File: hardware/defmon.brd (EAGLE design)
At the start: 50.8 x 48.1 mm, 18 parts, among them IC2 MEGA8-P, Q1 20MHz, X1 MAB5SH, X2 1503_09

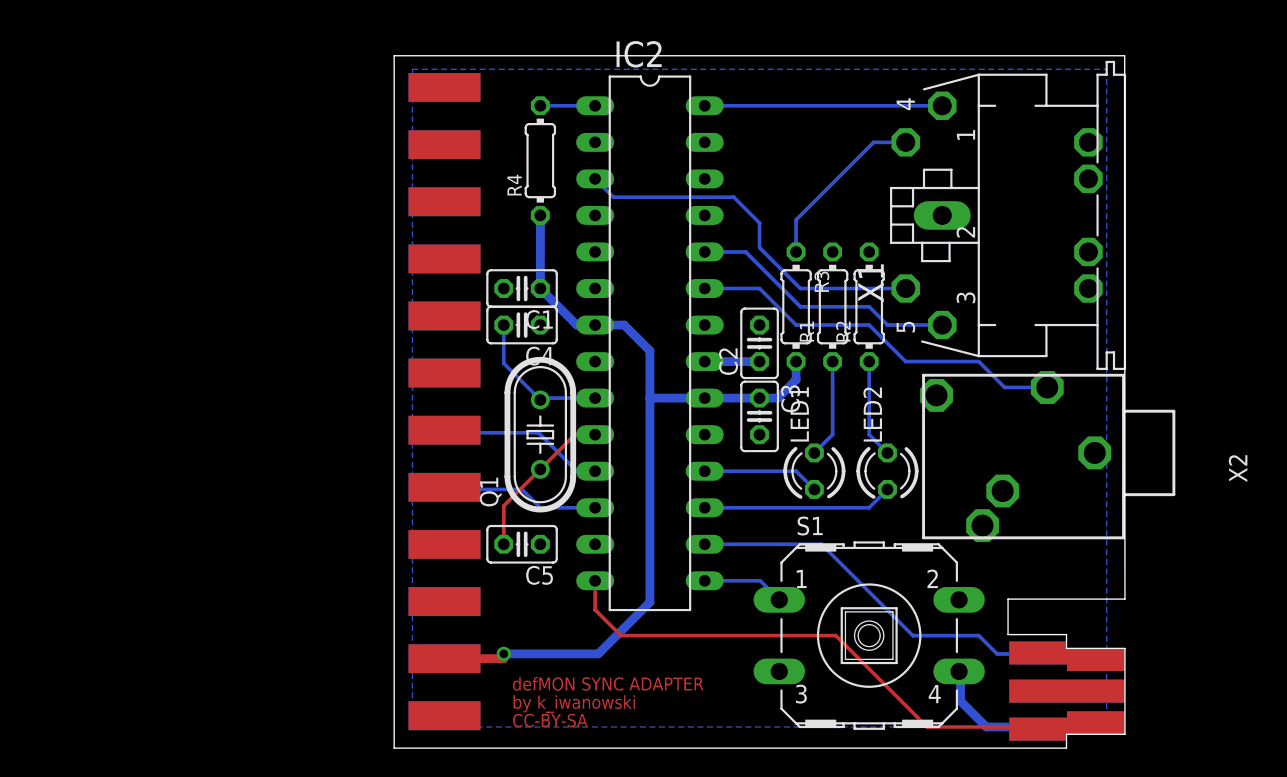
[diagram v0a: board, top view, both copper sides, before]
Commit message: Update cad files
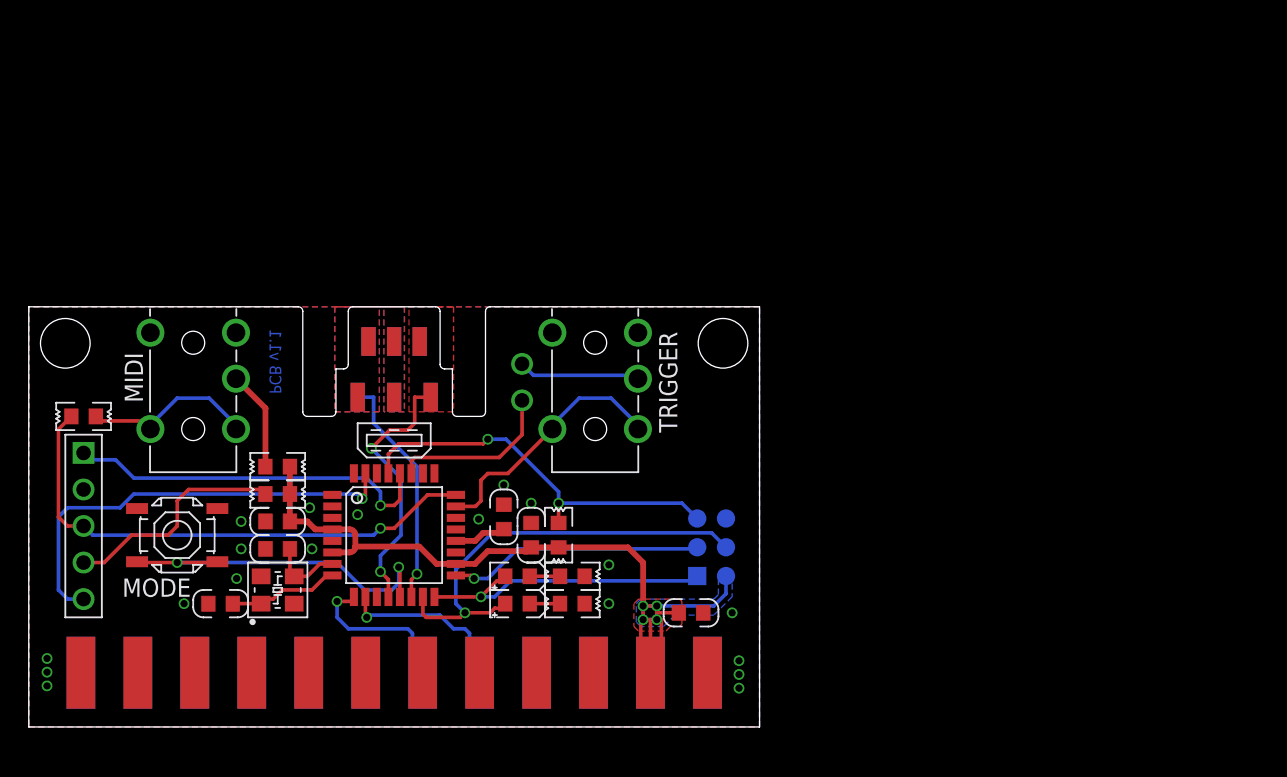
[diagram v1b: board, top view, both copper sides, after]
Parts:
- removed C1: 100nf, rcl:C025-025X050
- removed IC2: MEGA8-P, atmel:DIL28-3
- removed LED1, LED2: (no value), led:LED3MM
- removed S1: (no value), switch-omron:B3F-40XX
- removed X1: MAB5SH, con-hirschmann:MAB5SH
- removed X2: 1503_09, con-lumberg:1503_09
- added C6: 100n, rcl:C0603K
- added CONN2: DNP, GenMDMv2:ICSP_SMD_PROBE
- added CONN3: LINK_PORTFINAL, LinkPort by Jazz:DUAL_BAORD_LINK_FINAL
- added CU: 10uF, rcl:C0603K
- added DIN: 1X5, header by Jazz:1X5
- added IC1: MEGA8-AI_C16190, atmel:TQFP32-08
- added JP1: 2X1, header by Jazz:2X1
- added LED3, LED4: C2286, Led by Jazz:0603K
- added MIDI, TRIG: PJ313, GenMDMv200:PJ313D
- added R5, R6: 220Ohms, rcl:R0603
- added SW1: MODE, Switch by Jazz:TS5215A
- added U$3, U$8: (no value), Mount by Jazz:MOUNT4-40
- added U$9: (no value), Logos by Jazz:CATSKULL_PIXEL_MD
- C2, C3: value 100nf -> 100n; device rcl:C025-025X050 -> rcl:C0603K
- C4, C5: device rcl:C025-025X050 -> rcl:C0603K
- Q1: value 20MHz -> 20MHz_C172730; device crystal:HC49U-V -> GenMDMv200:SX3225
- R1, R2: value 220 -> 220ohms; device rcl:0204/7 -> rcl:R0603
- R3: value 220 -> 220Ohms; device rcl:0204/7 -> rcl:R0603
- R4: value 10k -> 10kOhms; device rcl:0204/7 -> rcl:R0603
- U$1: value GB -> (none); device connector:GB -> Logos by Jazz:JLCJLCJLCJLC
- U$2: value C64U -> CONNECTOR_C64UJ; device connector:C64U -> defmon:C64_USERPORT
- moved U$1 74.5 mm to (-24.3, 15.2), flipped to the bottom, turned to 270 degrees
- moved R2 55.1 mm to (-21.6, 22.9), turned to 180 degrees
- moved U$2 45.9 mm to (0.00, 0.00), turned to 0 degrees
- moved R1 40.1 mm to (-8.10, 19.4), turned to 0 degrees
- moved R3 38.3 mm to (-8.10, 17.5), turned to 0 degrees
- moved R4 26.1 mm to (11.4, 14.6)
- moved C4 23.0 mm to (-8.10, 13.7)
- moved C2 21.5 mm to (7.62, 15.9)
- moved C5 21.4 mm to (-12.1, 9.84)
- moved Q1 21.2 mm to (-8.10, 10.8), turned to 0 degrees
- moved C3 17.9 mm to (9.53, 14.6), turned to 90 degrees
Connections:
- removed net CLK: IC2.14, U$1.5
- removed net N$13: IC2.3, X1.5
- removed net PE: X1.PE, X1.PE@
- removed net S_OUT: IC2.16, U$1.2
- new net !RESET: CONN2.RST, IC1.29, R4.2
- new net +5V: C3.1, C6.1, CONN2.VCC, CU.1, IC1.18, IC1.4, IC1.6, R1.2, R3.2, R4.1, U$2.2
- new net GBCLK: CONN3.CLK1, CONN3.CLK2, IC1.12
- new net GBSOUT: CONN3.OUT1, CONN3.OUT2, IC1.14
- new net MISO: CONN2.MISO, IC1.16, LED3.A
- new net MOSI: CONN2.MOSI, IC1.15, LED4.A
- new net N$20: IC1.13, SW1.1, SW1.2
- new net N$7: LED4.C, R6.1
- new net PC5: DIN.P$1, IC1.28
- new net PD1: DIN.P$5, IC1.31
- new net SCK: CONN2.SCK, IC1.17
- net AREF: now also IC1.20; no longer IC2.21
- net EN: now also IC1.10; no longer IC2.12
- net GND: now also C4.2, C5.2, C6.2, CONN2.GND, CONN3.GND1, CONN3.GND2, CU.2, DIN.P$2, IC1.21, IC1.3, IC1.5, MIDI.2, MIDI.22, Q1.2, Q1.4, R5.2, R6.2, SW1.3, SW1.4, TRIG.2, TRIG.22; no longer C1.2, C4.1, C5.1, IC2.22, IC2.8, R1.2, R2.2, S1.3, S1.4, U$1.6, X1.2, X2.1
- net N$1: now also CONN3.VCC1, CONN3.VCC2; no longer LED2.K, R2.1
- net N$10: now also IC1.27, JP1.P$1; no longer C1.1, C3.1, IC2.20, IC2.7, R3.2, R4.1, U$2.2
- net N$11: now also C5.1, IC1.8; no longer C5.2, IC2.10
- net N$12: now also MIDI.3, R1.1; no longer IC2.1, R4.2
- net N$2: now also CONN3.SD1, CONN3.SD2; no longer LED1.K, R1.1
- net N$3: now also DIN.P$4; no longer X1.4
- net N$4: now also LED3.C, R5.1; no longer IC2.15, S1.1
- net N$5: now also CONN3.IN1, CONN3.IN2; no longer IC2.17, LED2.A
- net N$6: now also MIDI.4, MIDI.44, R2.1; no longer IC2.18, LED1.A
- net N$8: now also C4.1, IC1.7, Q1.3; no longer C4.2, IC2.9, Q1.2
- net N$9: now also JP1.P$2, TRIG.3; no longer IC2.28, X1.1
- net SYNC: now also IC1.9; no longer IC2.11
- net TRIG1: now also IC1.23, TRIG.4, TRIG.44; no longer IC2.23, X2.2
- net TRIG2: now also DIN.P$3, IC1.24, R2.2; no longer IC2.24, X1.3
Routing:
- net +5V: track 0.00 -> 64.7 mm, vias 0 -> 4
- net N$10: track 60.0 -> 11.7 mm, vias 1 -> 0
- net CLK: track 40.5 -> 0.00 mm
- net MOSI: track 0.00 -> 30.9 mm, vias 0 -> 1
- net PD1: track 0.00 -> 30.8 mm, vias 0 -> 1
- net S_OUT: track 30.7 -> 0.00 mm
- net !RESET: track 0.00 -> 27.4 mm, vias 0 -> 2
- net PC5: track 0.00 -> 26.1 mm, vias 0 -> 1
- net N$13: track 25.8 -> 0.00 mm
- net N$20: track 0.00 -> 25.2 mm, vias 0 -> 2
- net MISO: track 0.00 -> 21.1 mm, vias 0 -> 1
- net GBCLK: track 0.00 -> 18.7 mm, vias 0 -> 2
- net TRIG2: track 18.6 -> 36.7 mm, vias 0 -> 1
- net SCK: track 0.00 -> 17.8 mm, vias 0 -> 1
- net GBSOUT: track 0.00 -> 16.4 mm, vias 0 -> 1
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- added copper zone on layer 1, net +5V
- added copper zone on layer 16, net +5V
- added copper zone on layer 1, net GBCLK
- added copper zone on layer 16, net GBSOUT
- added copper zone on layer 1, net GND
- added copper zone on layer 1, net N$1
- added copper zone on layer 16, net N$2
- added copper zone on layer 1, net N$5
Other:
- board size 50.8 x 48.1 mm -> 50.8 x 29.2 mm
- board text added: "MIDI"
- board text added: "MODE"
- board text added: "PCB v1.1"
- board text added: "TRIGGER"
- board text added: "defMON SYNC ADAPTER by k_iwanowski CC-BY-SA"
- board text removed: "CC-BY-SA"
- board text removed: "by k_iwanowski"
- board text removed: "defMON SYNC ADAPTER"
